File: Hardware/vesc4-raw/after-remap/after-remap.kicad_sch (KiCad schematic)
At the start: 26 parts, among them K1 SERVO, P1 HALL/Encoder, P101 CANBUS, P3 PWR_COMM, P4 IN+, P5 IN-, P6 MOTOR1, P7 MOTOR2, P9 MOTOR3

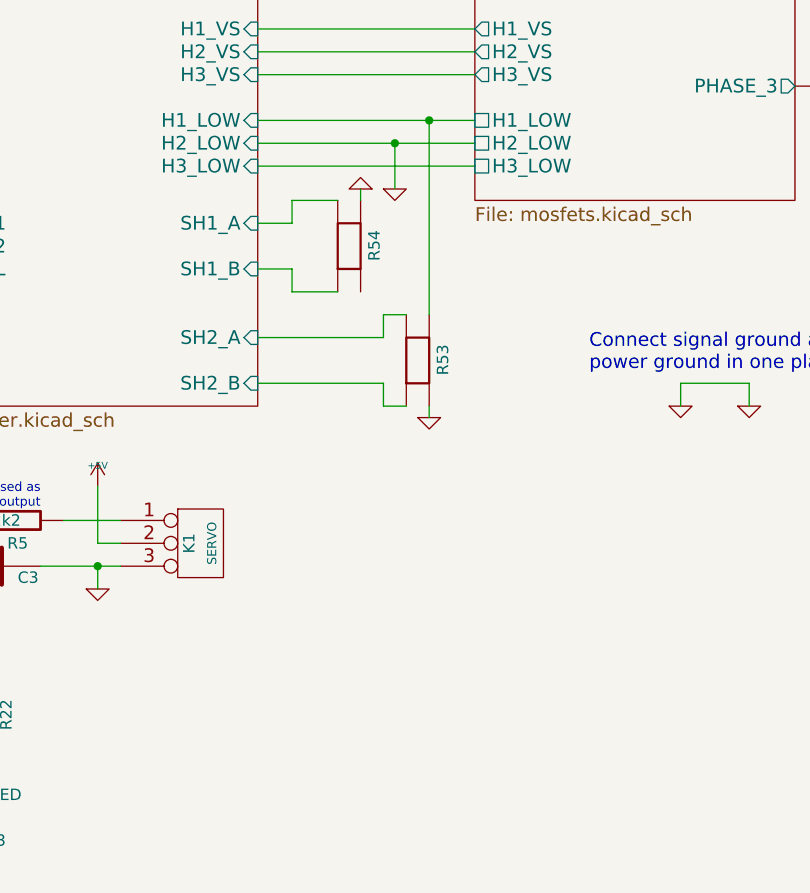
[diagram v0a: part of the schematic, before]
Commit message: ganti shunt
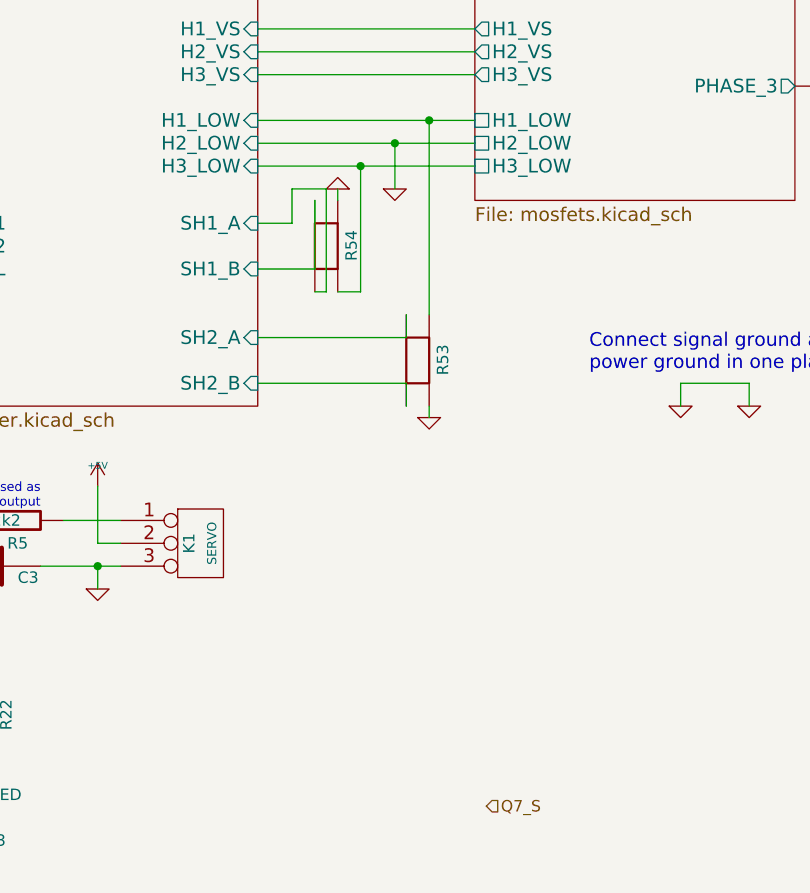
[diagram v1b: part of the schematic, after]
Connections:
- net Mosfet driver/H3_LOW: now also R54.3
- net Mosfet driver/SH1_A: now also R54.1; no longer R54.2
- net Mosfet driver/SH1_B: now also R54.2; no longer R54.1
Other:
- moved on the sheet: R54
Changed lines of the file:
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@@
 	)
 	(junction
+		(at 207.01 101.6)
+		(diameter 0)
+		(color 0 0 0 0)
+	)
+	(junction
 		(at 16.51 82.55)
 		(diameter 0)
@@
 	(wire
 		(pts
-			(xy 199.39 113.03) (xy 195.58 113.03)
+			(xy 195.58 113.03) (xy 201.93 113.03)
 		)
 		(stroke
@@
 	(wire
 		(pts
-			(xy 207.01 104.14) (xy 207.01 105.41)
+			(xy 195.58 86.36) (xy 219.71 86.36)
 		)
 		(stroke
@@
 	(wire
 		(pts
-			(xy 195.58 86.36) (xy 219.71 86.36)
+			(xy 204.47 105.41) (xy 204.47 104.14)
 		)
 		(stroke
@@
 	(wire
 		(pts
+			(xy 199.39 104.14) (xy 203.2 104.14)
+		)
+		(stroke
+			(width 0)
+			(type default)
+		)
+	)
+	(wire
+		(pts
+			(xy 207.01 115.57) (xy 207.01 101.6)
+		)
+		(stroke
+			(width 0)
+			(type default)
+		)
+	)
+	(wire
+		(pts
 			(xy 34.29 74.93) (xy 54.61 74.93)
 		)
@@
 	(wire
 		(pts
-			(xy 199.39 105.41) (xy 204.47 105.41)
+			(xy 231.14 38.1) (xy 231.14 35.56)
 		)
 		(stroke
@@
 	(wire
 		(pts
-			(xy 231.14 38.1) (xy 231.14 35.56)
+			(xy 203.2 104.14) (xy 203.2 115.57)
 		)
 		(stroke
@@
 	(wire
 		(pts
-			(xy 147.32 140.97) (xy 160.02 140.97)
+			(xy 199.39 104.14) (xy 199.39 107.95)
 		)
 		(stroke
@@
 	(wire
 		(pts
-			(xy 147.32 97.79) (xy 157.48 97.79)
+			(xy 147.32 140.97) (xy 160.02 140.97)
 		)
 		(stroke
@@
 	(wire
 		(pts
-			(xy 209.55 118.11) (xy 212.09 118.11)
+			(xy 147.32 97.79) (xy 157.48 97.79)
 		)
 		(stroke
@@
 	(wire
 		(pts
-			(xy 199.39 107.95) (xy 199.39 105.41)
-		)
-		(stroke
-			(width 0)
-			(type default)
-		)
-	)
-	(wire
-		(pts
 			(xy 199.39 107.95) (xy 195.58 107.95)
 		)
@@
 	(wire
 		(pts
-			(xy 195.58 120.65) (xy 209.55 120.65)
-		)
-		(stroke
-			(width 0)
-			(type default)
-		)
-	)
-	(wire
-		(pts
-			(xy 209.55 128.27) (xy 212.09 128.27)
-		)
-		(stroke
-			(width 0)
-			(type default)
-		)
-	)
-	(wire
-		(pts
-			(xy 199.39 115.57) (xy 204.47 115.57)
+			(xy 195.58 120.65) (xy 212.09 120.65)
 		)
 		(stroke
@@
 	(wire
 		(pts
+			(xy 212.09 120.65) (xy 212.09 118.11)
+		)
+		(stroke
+			(width 0)
+			(type default)
+		)
+	)
+	(wire
+		(pts
 			(xy 16.51 85.09) (xy 16.51 82.55)
 		)
@@
 	(wire
 		(pts
-			(xy 195.58 125.73) (xy 209.55 125.73)
+			(xy 195.58 125.73) (xy 212.09 125.73)
 		)
 		(stroke
@@
 	(wire
 		(pts
+			(xy 201.93 113.03) (xy 201.93 105.41)
+		)
+		(stroke
+			(width 0)
+			(type default)
+		)
+	)
+	(wire
+		(pts
 			(xy 35.56 85.09) (xy 40.64 85.09)
 		)
@@
 	(wire
 		(pts
-			(xy 209.55 120.65) (xy 209.55 118.11)
+			(xy 160.02 146.05) (xy 161.29 146.05)
 		)
 		(stroke
@@
 	(wire
 		(pts
-			(xy 160.02 146.05) (xy 161.29 146.05)
+			(xy 36.83 140.97) (xy 82.55 140.97)
 		)
 		(stroke
@@
 	(wire
 		(pts
-			(xy 36.83 140.97) (xy 82.55 140.97)
+			(xy 43.18 57.15) (xy 43.18 60.96)
 		)
 		(stroke
@@
 	(wire
 		(pts
-			(xy 43.18 57.15) (xy 43.18 60.96)
+			(xy 72.39 119.38) (xy 82.55 119.38)
 		)
 		(stroke
@@
 	(wire
 		(pts
-			(xy 72.39 119.38) (xy 82.55 119.38)
+			(xy 177.8 146.05) (xy 177.8 148.59)
 		)
 		(stroke
@@
 	(wire
 		(pts
-			(xy 177.8 146.05) (xy 177.8 148.59)
+			(xy 147.32 63.5) (xy 157.48 63.5)
 		)
 		(stroke
@@
 	(wire
 		(pts
-			(xy 147.32 63.5) (xy 157.48 63.5)
+			(xy 35.56 90.17) (xy 35.56 85.09)
 		)
 		(stroke
@@
 	(wire
 		(pts
-			(xy 35.56 90.17) (xy 35.56 85.09)
+			(xy 207.01 101.6) (xy 219.71 101.6)
 		)
 		(stroke
@@
 	(wire
 		(pts
-			(xy 177.8 146.05) (xy 180.34 146.05)
+			(xy 212.09 125.73) (xy 212.09 128.27)
 		)
 		(stroke
@@
 	(wire
 		(pts
-			(xy 209.55 125.73) (xy 209.55 128.27)
+			(xy 177.8 146.05) (xy 180.34 146.05)
 		)
 		(stroke
@@
 	(wire
 		(pts
-			(xy 199.39 113.03) (xy 199.39 115.57)
+			(xy 250.19 125.73) (xy 250.19 128.27)
 		)
 		(stroke
@@
 	(wire
 		(pts
-			(xy 250.19 125.73) (xy 250.19 128.27)
+			(xy 203.2 115.57) (xy 201.93 115.57)
 		)
 		(stroke
@@
 	(wire
 		(pts
-			(xy 58.42 54.61) (xy 59.69 54.61)
+			(xy 195.58 101.6) (xy 207.01 101.6)
 		)
 		(stroke
@@
 	(wire
 		(pts
-			(xy 214.63 96.52) (xy 219.71 96.52)
+			(xy 58.42 54.61) (xy 59.69 54.61)
 		)
 		(stroke
@@
 	(wire
 		(pts
-			(xy 171.45 146.05) (xy 177.8 146.05)
+			(xy 214.63 96.52) (xy 219.71 96.52)
 		)
 		(stroke
@@
 	(wire
 		(pts
-			(xy 195.58 101.6) (xy 219.71 101.6)
+			(xy 171.45 146.05) (xy 177.8 146.05)
 		)
 		(stroke
@@
 	(wire
 		(pts
+			(xy 204.47 115.57) (xy 207.01 115.57)
+		)
+		(stroke
+			(width 0)
+			(type default)
+		)
+	)
+	(wire
+		(pts
 			(xy 149.86 149.86) (xy 149.86 156.21)
 		)
@@
 		)
 	)
+	(hierarchical_label "Q7_S"
+		(shape input)
+		(at 220.98 172.72 0)
+		(effects
+			(font
+				(size 1.27 1.27)
+			)
+			(justify left)
+		)
+	)
 	(symbol
 		(lib_name "CONN_6_2")
@@
 		(lib_name "GND-RESCUE-BLDC_4_17")
 		(lib_id "vesc4-legacy:GND-RESCUE-BLDC_4_17")
-		(at 207.01 104.14 180)
+		(at 204.47 104.14 180)
 		(unit 1)
 		(exclude_from_sim no)
@@
 		(dnp no)
 		(property "Reference" "#PWR020"
-			(at 207.01 104.14 0)
+			(at 204.47 104.14 0)
 			(effects
 				(font
@@
 		)
 		(property "Value" "GND"
-			(at 207.01 102.362 0)
+			(at 204.47 102.362 0)
 			(effects
 				(font
@@
 		)
 		(property "Footprint" ""
-			(at 207.01 104.14 0)
+			(at 204.47 104.14 0)
 			(effects
 				(font
@@
 		)
 		(property "Datasheet" ""
-			(at 207.01 104.14 0)
+			(at 204.47 104.14 0)
 			(effects
 				(font
@@
 		)
 		(property "Description" ""
-			(at 207.01 104.14 0)
+			(at 204.47 104.14 0)
 			(effects
 				(font
@@
 	(symbol
 		(lib_id "Library:WSLP27262L000FEA")
-		(at 205.74 110.49 90)
+		(at 203.2 110.49 90)
 		(unit 1)
 		(exclude_from_sim no)
@@
 		(dnp no)
 		(property "Reference" "R54"
-			(at 208.534 108.712 0)
+			(at 205.994 108.712 0)
 			(effects
 				(font
@@
 		)
 		(property "Value" "WSLP27262L000FEA"
-			(at 208.28 111.7599 90)
+			(at 205.74 111.7599 90)
 			(effects
 				(font
@@
 		)
 		(property "Footprint" "Library:C2076510"
-			(at 205.74 110.49 0)
+			(at 203.2 110.49 0)
 			(effects
 				(font
@@
 		)
 		(property "Datasheet" ""
-			(at 205.74 110.49 0)
+			(at 203.2 110.49 0)
 			(effects
 				(font
@@
 		)
 		(property "Description" ""
-			(at 205.74 110.49 0)
+			(at 203.2 110.49 0)
 			(effects
 				(font
@@
 		)
 		(property "Manufacturer Part" "WSLP27262L000FEA"
-			(at 205.74 110.49 0)
+			(at 203.2 110.49 0)
 			(effects
 				(font
@@
 		)
 		(property "Manufacturer" "VISHAY(威世)"
-			(at 205.74 110.49 0)
+			(at 203.2 110.49 0)
 			(effects
 				(font
@@
 		)
 		(property "Supplier Part" "C2076510"
-			(at 205.74 110.49 0)
+			(at 203.2 110.49 0)
 			(effects
 				(font
@@
 		)
 		(property "Supplier" "LCSC"
-			(at 205.74 110.49 0)
+			(at 203.2 110.49 0)
 			(effects
 				(font

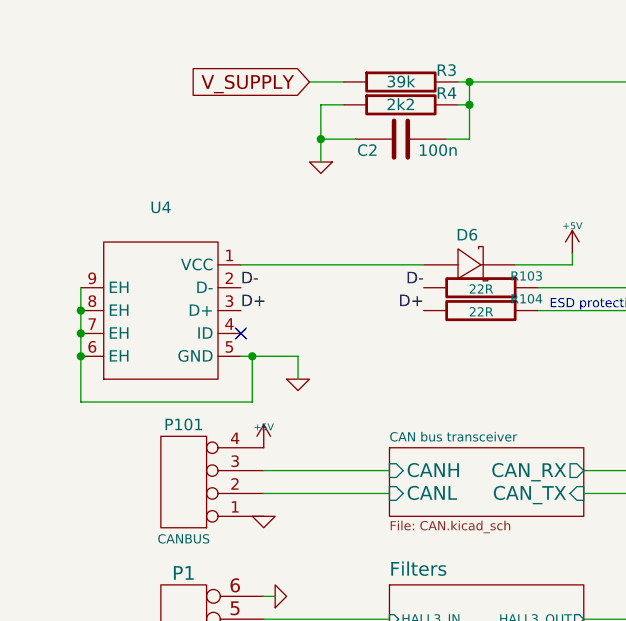
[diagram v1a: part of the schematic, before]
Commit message: changed USB
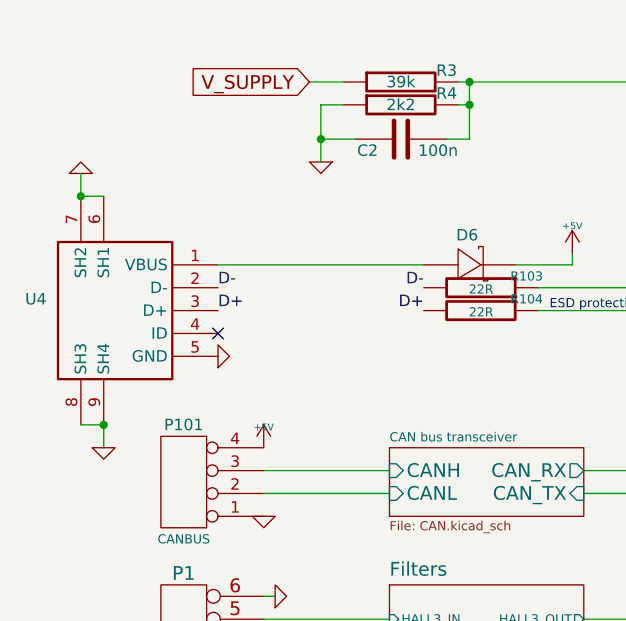
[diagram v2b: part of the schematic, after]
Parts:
- removed U4: ~, EasyEDA_Lib:MICRO-USB-SMD_MICROUSB-5P-M, symbol EasyEDA_Lib:MICRO USB 5P贴板公头四脚贴带卡勾
- added U4: MICROQTJ, symbol Library:MICROQTJ
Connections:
- net D+: now also U4.3 (D+)
- net D-: now also U4.2 (D-)
- net GND: now also U4.5 (GND), U4.6 (SH1), U4.7 (SH2), U4.8 (SH3), U4.9 (SH4)
- net at D6.2 (A): now also U4.1 (VBUS)

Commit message: sebelum ganti kapasitor 1206
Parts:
- U4: footprint (none) -> Library:MICRO-USB-SMD_MICROQTJ-5P
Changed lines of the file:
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@@
 			)
 		)
-		(property "Footprint" ""
+		(property "Footprint" "Library:MICRO-USB-SMD_MICROQTJ-5P"
 			(at 24.13 80.01 0)
 			(effects
